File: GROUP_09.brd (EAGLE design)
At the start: 83.8 x 55.9 mm, 29 parts, among them J1 POWER_JACKPTH_LOCK, U1 +12v, U3 TCA9546ATSSOP16, U4 TMUX1208QNF

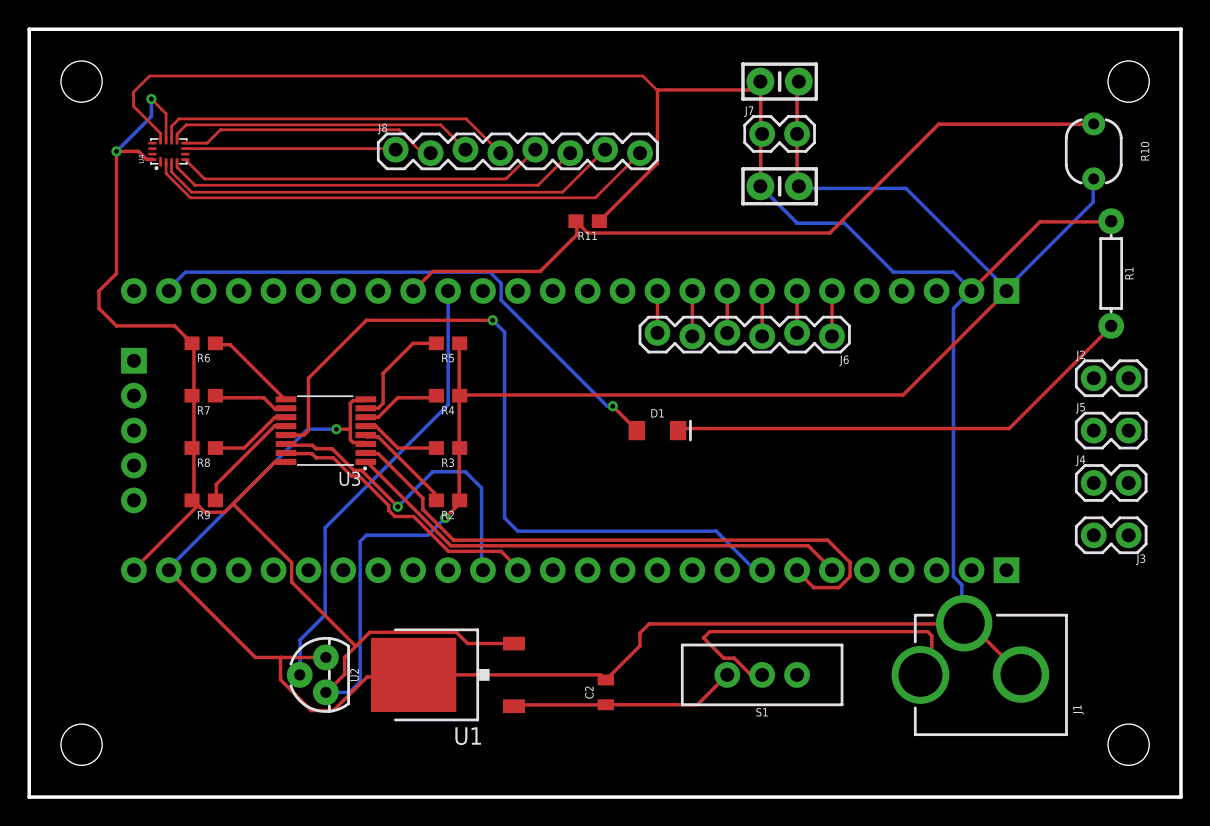
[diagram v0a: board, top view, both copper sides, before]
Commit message: Final version
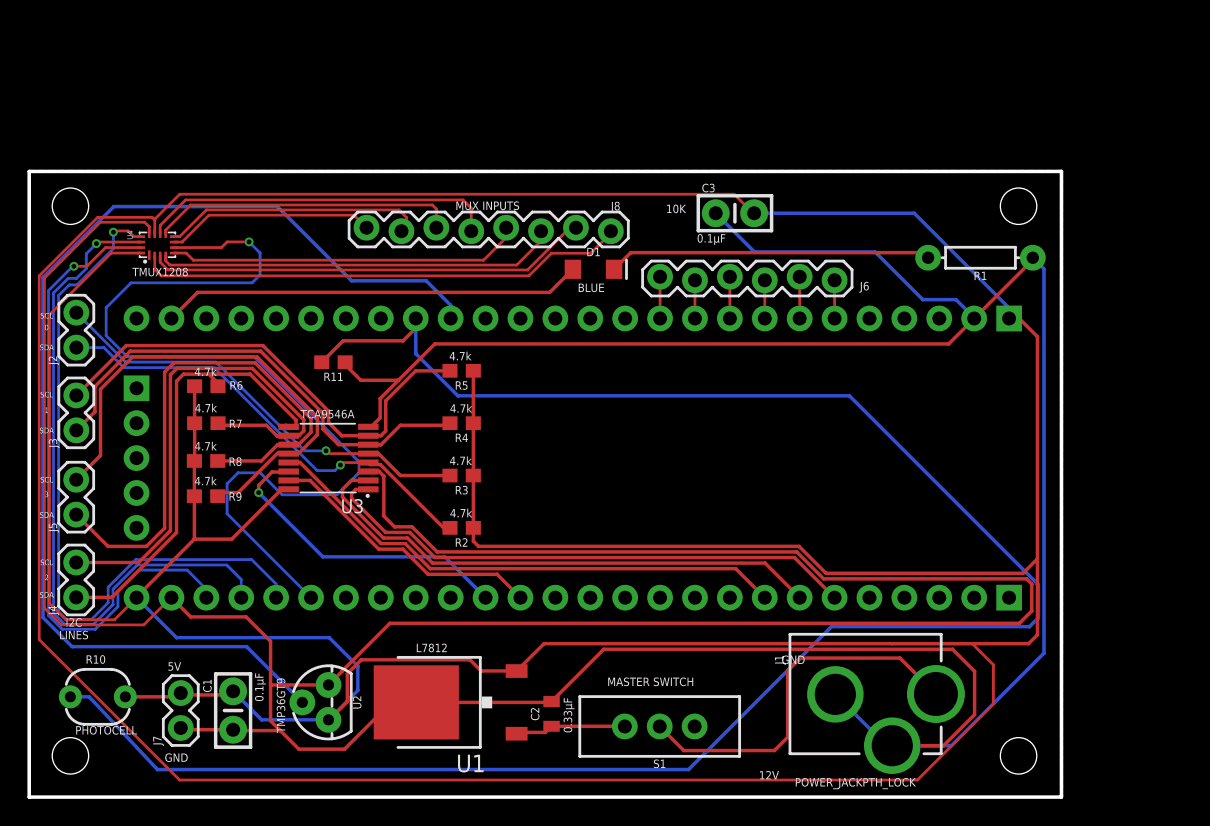
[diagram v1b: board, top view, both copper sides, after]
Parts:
- J2, J3, J4, J5, J6, J7, J8, S1, U2: value (none) -> (none)
- moved R10 82.6 mm to (4.99, 7.29), turned to 0 degrees
- moved J3 77.0 mm to (3.43, 26.7), turned to 90 degrees
- moved J4 74.5 mm to (3.42, 14.5), turned to 90 degrees
- moved J5 74.3 mm to (3.42, 20.6), turned to 90 degrees
- moved J2 74.1 mm to (3.43, 32.7), turned to 90 degrees
- moved J7 60.5 mm to (11.0, 5.03), turned to 90 degrees
- moved C1 55.1 mm to (14.8, 6.30), turned to 270 degrees
- moved J1 26.7 mm to (52.1, 7.50), turned to 270 degrees
- moved R11 21.2 mm to (22.1, 31.6)
- moved D1 12.6 mm to (41.1, 38.4)
- moved C3 10.1 mm to (51.4, 42.5)
- moved R1 9.58 mm to (69.2, 39.2), turned to 180 degrees
- moved S1 8.35 mm to (45.9, 5.14)
- moved U4 6.85 mm to (9.33, 40.2)
- moved J8 6.07 mm to (24.5, 41.3)
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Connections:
- net N$12 renamed MIC_0.5
- net N$13 renamed MIC_0.4
- net N$14 renamed MIC_0.3
- net N$15 renamed MIC_0.2
- net N$16 renamed MIC_0.1
- net N$17 renamed MIC_0.0
- net N$18 renamed MUX_S8
- net N$19 renamed MUX_S7
- net N$20 renamed MUX_S6
- net N$21 renamed MUX_S5
- net N$22 renamed MUX_S4
- net N$23 renamed MUX_S3
- net N$24 renamed MUX_S2
- net N$25 renamed MUX_S1
- removed net MUX_A0/1.3C: U4.15
- removed net MUX_A0/2.3C: CY8CKIT059-TARGET.24
- removed net MUX_A1/1.4C: U4.14
- removed net MUX_A1/2.3C: CY8CKIT059-TARGET.23
- removed net MUX_A2/1.4C: U4.13
- removed net MUX_A2/2.3C: CY8CKIT059-TARGET.22
- removed net MUX_OUT/1.4C: U4.6
- removed net MUX_OUT/2.5C: CY8CKIT059-TARGET.21
- removed net N$1: R2.2, U3.4
- removed net N$10: R6.1, U3.9
- removed net N$3: R3.2, U3.5
- removed net N$4: R4.2, U3.6
- removed net N$5: R5.2, U3.7
- removed net N$7: R9.1, U3.12
- removed net N$8: R8.1, U3.11
- removed net N$9: R7.1, U3.10
- new net MUX_A0: CY8CKIT059-TARGET.24, U4.15
- new net MUX_A1: CY8CKIT059-TARGET.23, U4.14
- new net MUX_A2: CY8CKIT059-TARGET.22, U4.13
- new net MUX_OUT: CY8CKIT059-TARGET.21, U4.6
- net I2C_SCL_0: now also R3.2, U3.5
- net I2C_SCL_1: now also R5.2, U3.7
- net I2C_SCL_2: now also R7.1, U3.10
- net I2C_SCL_3: now also R9.1, U3.12
- net I2C_SDA_0: now also R2.2, U3.4
- net I2C_SDA_1: now also R4.2, U3.6
- net I2C_SDA_2: now also R6.1, U3.9
- net I2C_SDA_3: now also R8.1, U3.11
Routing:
- net 5V: track 202.3 -> 428.6 mm, vias 3 -> 0
- net GND: track 224.4 -> 374.5 mm, vias 1 -> 0
- net PHOTO_OUT: track 55.8 -> 143.1 mm
- net MUX_OUT: track 0.00 -> 67.7 mm, vias 0 -> 1
- net MUX_A2: track 0.00 -> 52.1 mm, vias 0 -> 1
- net MUX_A1: track 0.00 -> 50.1 mm, vias 0 -> 1
- net TEMP_OUT: track 32.4 -> 81.9 mm
- net MUX_A0: track 0.00 -> 47.2 mm, vias 0 -> 1
- net I2C_SDA_3: track 0.00 -> 40.6 mm
- net I2C_SCL_2: track 0.00 -> 38.2 mm
- net I2C_SCL_3: track 0.00 -> 36.3 mm
- net I2C_SCL_1: track 0.00 -> 35.1 mm
- net I2C_SDA_1: track 0.00 -> 34.8 mm
- net I2C_SDA_2: track 0.00 -> 33.4 mm
- net I2C_SDA_0: track 0.00 -> 33.3 mm, vias 0 -> 1
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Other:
- board size 83.8 x 55.9 mm -> 75.1 x 45.5 mm
- board text added: "0"
- board text added: "0.1µF"
- board text added: "0.33µF"
- board text added: "1"
- board text added: "10K"
- board text added: "12V"
- board text added: "2"
- board text added: "3"
- board text added: "4.7k"
- board text added: "5V"
- board text added: "BLUE"
- board text added: "C1"
- board text added: "C3"
- board text added: "CY8CKIT059-TARGET"
- board text added: "GND"
- board text added: "I2C LINES"
- board text added: "L7812"
- board text added: "MASTER SWITCH"
- board text added: "MUX INPUTS"
- board text added: "PHOTOCELL"
- board text added: "POWER_JACKPTH_LOCK"
- board text added: "SCL"
- board text added: "SDA"
- board text added: "TCA9546A"
- board text added: "TMP36GT9"
- board text added: "TMUX1208"
